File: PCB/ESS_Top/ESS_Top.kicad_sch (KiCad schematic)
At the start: 3 parts, among them J1 Conn_01x15, J2 Conn_01x15

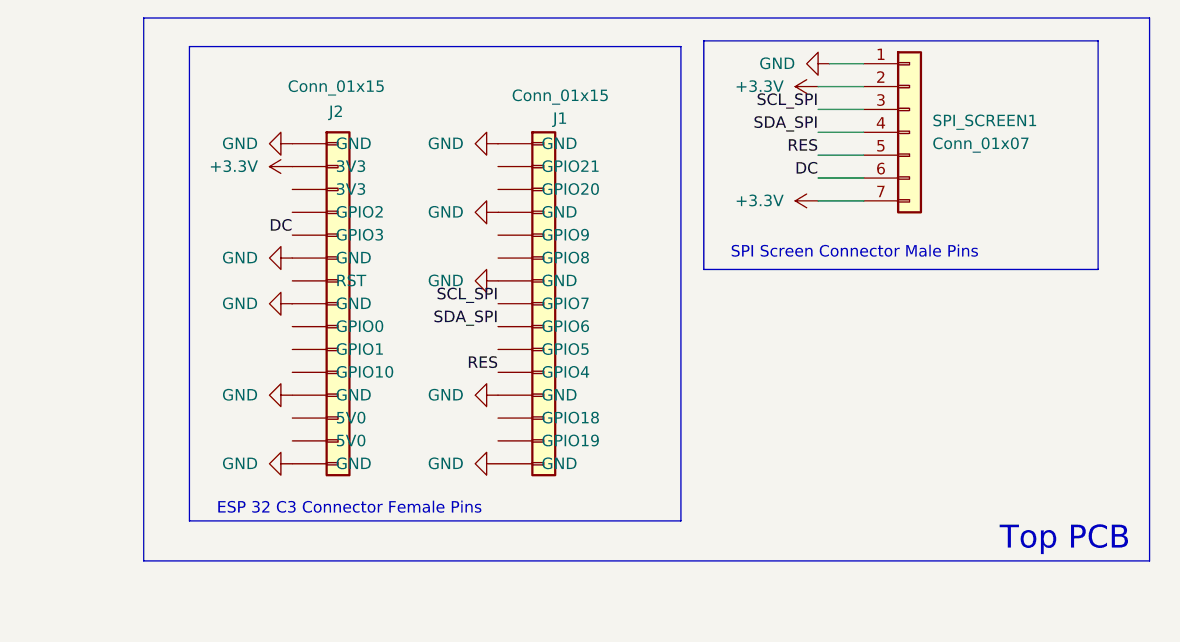
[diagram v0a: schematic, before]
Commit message: made kicad files cleaner?
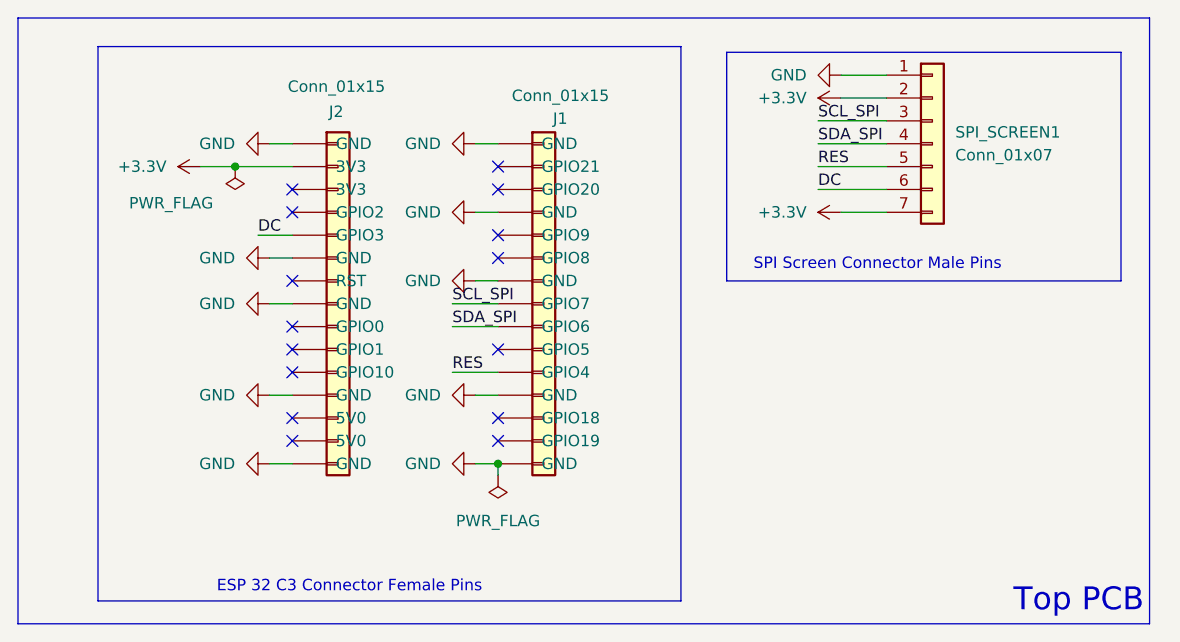
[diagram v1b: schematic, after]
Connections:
- no-connect marks 0 -> 15
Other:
- moved on the sheet: SPI_SCREEN1
